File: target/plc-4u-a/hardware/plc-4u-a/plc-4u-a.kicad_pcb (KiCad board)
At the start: 2 copper layers, 363.5 x 84 mm, 205 parts, among them J1 Screw_Terminal_01x02, J10 AUX_INS, J11 X Leds Btns, J12 S3 S5 LEDs, J13 Valve control in, J14 Leak sensors, J15 I2C, J16 I2C, J17 TA_C, J18 X leds btns, J19 Valve leds, J2 Screw_Terminal_01x02, J20 Valve leds, J21 Leak sensors, J22 Valve control in, J23 S3 S5 LEDs, J24 S4 S6 LEDs, J25 S3 S5 LEDs, J26 S4 S6 LEDs, J27 S3BTN, J28 S4BTN, J29 S5BTN, J3 Screw_Terminal_01x02, J30 S6BTN, J31 S3BTN, J32 S4BTN, J33 S5BTN, J34 S6BTN, J35 PWR_OUT, J36 Sensors AB, J37 Sensors CD, J38 PWR_OUT, J39 Leak sensors, J4 Screw_Terminal_01x02, J40 Leak sensors, J41 TA_C, J42 TB_C, J43 TC_C, J44 TD_C, J45 TB_C, J46 TC_C, J47 TD_C, J48 S3 S5 LEDs, J49 S1 S2 LEDs, J5 Screw_Terminal_01x02, J50 S1 S2 BTNS, J51 X0, J52 U8 IN, J53 X0, J54 X9 IN, J55 AVR-ISP-10, J56 U17 OUT, J57 U8 OUT, J58 U17 OUT, J59 U8 OUT, J6 V_ST_HWS, J60 GND, J61 GND, J62 VCC, J63 VCC, J64 SIM800, J65 RES_IN, J66 SELF_PWR_IN, J67 VDD VSS, J68 VDD VSS, J69 VDD, J7 V_ST_CWS, J70 VDD, J71 RES_OUT, J72 VSS, J73 VSS, J74 VSS, J75 VSS, J76 VSS, J77 VDD, J78 VDD, J79 NC, J8 W_CT_HWS, J80 NC, J81 NC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

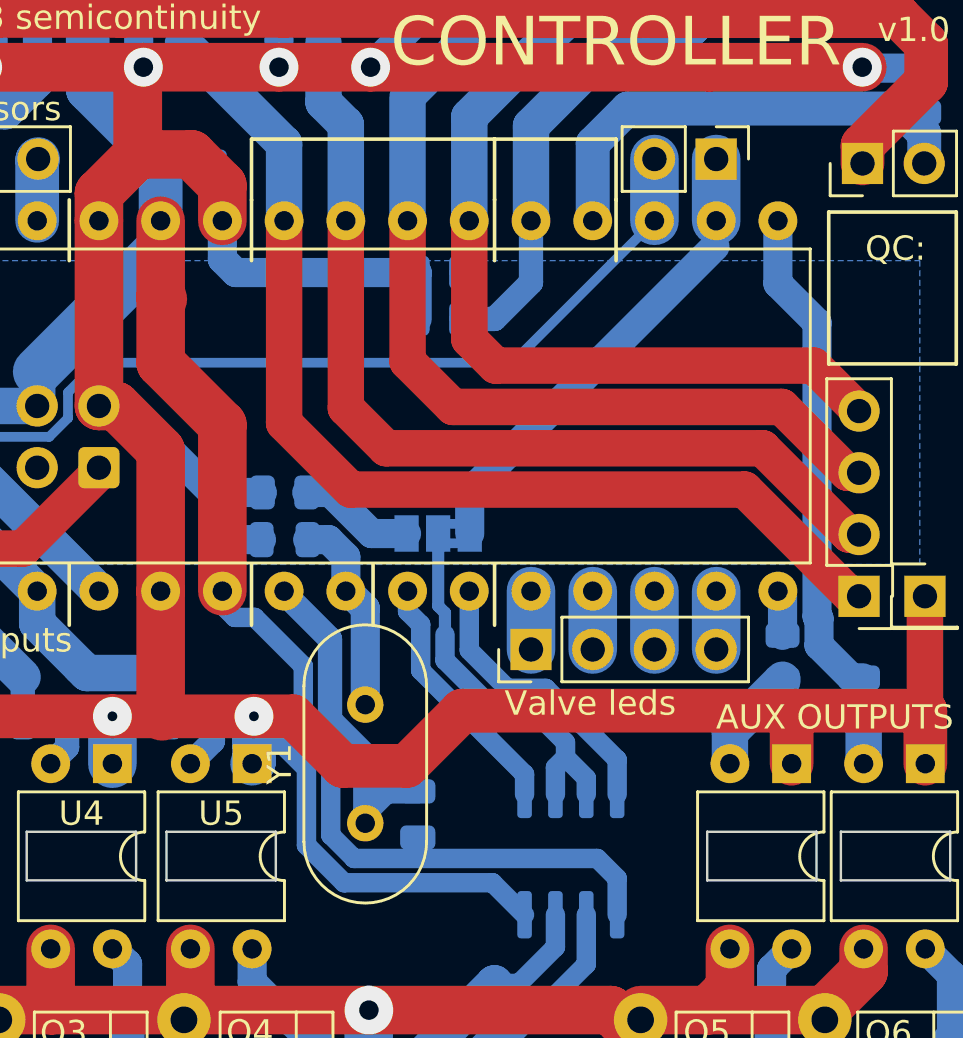
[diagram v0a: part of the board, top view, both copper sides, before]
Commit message: plc-4u-a += pcb update
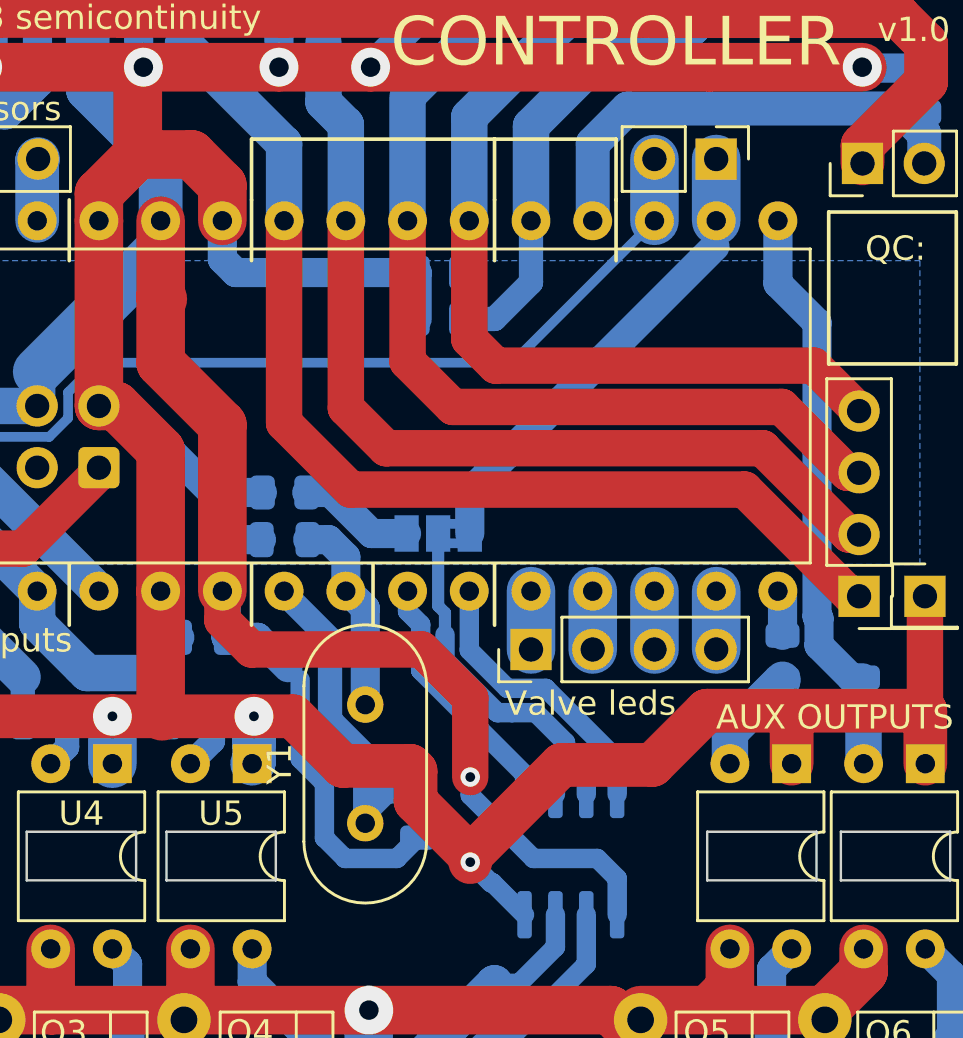
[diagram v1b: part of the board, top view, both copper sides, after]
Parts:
- added C3: C, Capacitor_SMD:C_0805_2012Metric, B.Cu at (99.8, 86.0)
- J71: value RES_OUT -> RESERVED_OUT
- moved C1 19.4 mm to (100.5, 105.5), turned to 0 degrees
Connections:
- net /Middle board/SDA renamed /Middle board/RXD
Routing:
- net /VSS: track 214.4 -> 230.8 mm, vias 0 -> 1
- net /VDD: track 209.4 -> 203.0 mm, vias 11 -> 12
- net unconnected-(J19-Pad4): track 2.40 -> 0.00 mm
- net unconnected-(J19-Pad2): track 0.00 -> 2.40 mm
- net unconnected-(J19-Pad1): track 2.40 -> 0.00 mm
- net /PD5: track 0.00 -> 2.40 mm
- net /PD3: track 2.40 -> 0.00 mm
- net /PD2: track 0.00 -> 2.40 mm
